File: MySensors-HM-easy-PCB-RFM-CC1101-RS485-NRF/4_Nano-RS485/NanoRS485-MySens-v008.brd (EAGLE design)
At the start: 25 x 38.7 mm, 47 parts, among them IC1 ATSHA204A, IC2 AT25DF512C-SSHN-B, IC3 REG1117, IC31 ATMEGA168-TQFP, X2 1751264, Y2 8MHZ

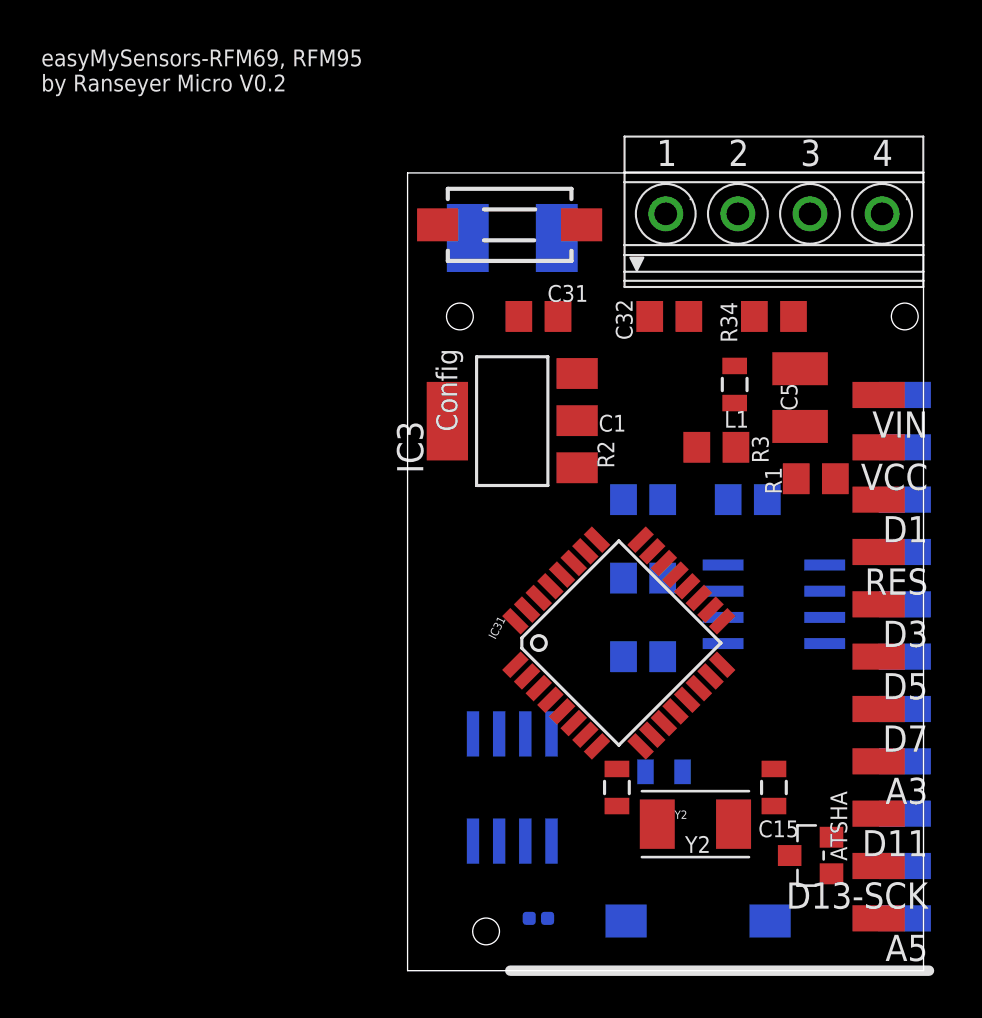
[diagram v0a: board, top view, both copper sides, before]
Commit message: update
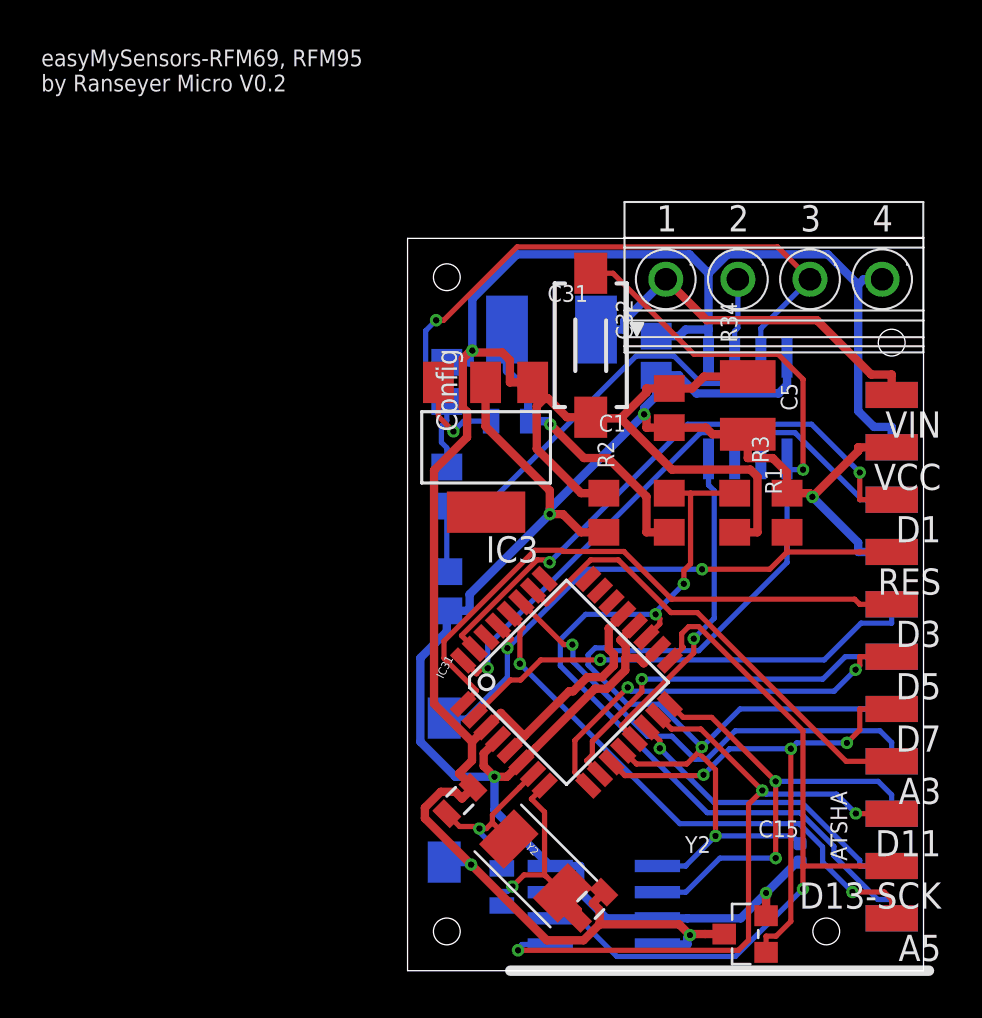
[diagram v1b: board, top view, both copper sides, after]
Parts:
- moved R7 15.7 mm to (1.91, 28.6), turned to 90 degrees
- moved C10 14.6 mm to (12.1, 29.8), turned to 270 degrees
- moved RESET 13.9 mm to (1.78, 8.76), turned to 90 degrees
- moved R2 13.1 mm to (19.1, 5.71), turned to 0 degrees
- moved L1 11.1 mm to (4.95, 26.7), flipped to the bottom, turned to 0 degrees
- moved C15 10.6 mm to (8.89, 3.17), turned to 225 degrees
- moved C32 10.0 mm to (9.53, 22.2), turned to 90 degrees
- moved R4 9.66 mm to (4.57, 4.06), turned to 90 degrees
- moved RS485 9.61 mm to (16.5, 27.3), turned to 90 degrees
- moved R5 9.55 mm to (1.91, 23.5), turned to 90 degrees
- moved R6 9.55 mm to (1.91, 18.4), turned to 90 degrees
- moved R34 9.55 mm to (18.4, 22.2), turned to 270 degrees
- moved Y2 8.01 mm to (6.22, 5.08), turned to 315 degrees
- moved C31 7.75 mm to (12.7, 27.3), turned to 90 degrees
- moved C14 7.65 mm to (2.54, 8.26), turned to 225 degrees
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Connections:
- removed net IN: F1.P$2
- removed net UREG: F1.P$1
- new net VIN-FUSED: F1.P$1, L1.1, R1.1
- net A: now also X2.2
- net B: now also X2.3
- net GND: now also X2.4
- net VIN: now also F1.P$2, X2.1; no longer L1.1, R1.1
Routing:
- net GND: track 0.00 -> 140.2 mm, vias 0 -> 3
- net VCC: track 0.00 -> 106.4 mm, vias 0 -> 5
- net D8: track 0.00 -> 68.5 mm, vias 0 -> 3
- net A6: track 0.00 -> 39.6 mm, vias 0 -> 2
- net D13_SCK: track 0.00 -> 36.1 mm, vias 0 -> 1
- net D11_MOSI: track 0.00 -> 34.0 mm, vias 0 -> 3
- net B: track 0.00 -> 33.5 mm, vias 0 -> 1
- net D2_INT0: track 0.00 -> 30.5 mm, vias 0 -> 1
- net D3: track 0.00 -> 28.6 mm
- net D1-TXD: track 0.00 -> 28.4 mm, vias 0 -> 2
- net RESET: track 0.00 -> 28.3 mm, vias 0 -> 2
- net A5: track 0.00 -> 26.9 mm, vias 0 -> 2
- net D7-ATSHA: track 0.00 -> 26.5 mm, vias 0 -> 3
- net A: track 0.00 -> 25.9 mm
- net D12_MISO: track 0.00 -> 23.7 mm, vias 0 -> 2
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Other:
- board size 25 x 38.7 mm -> 25 x 35.5 mm

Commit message: Update
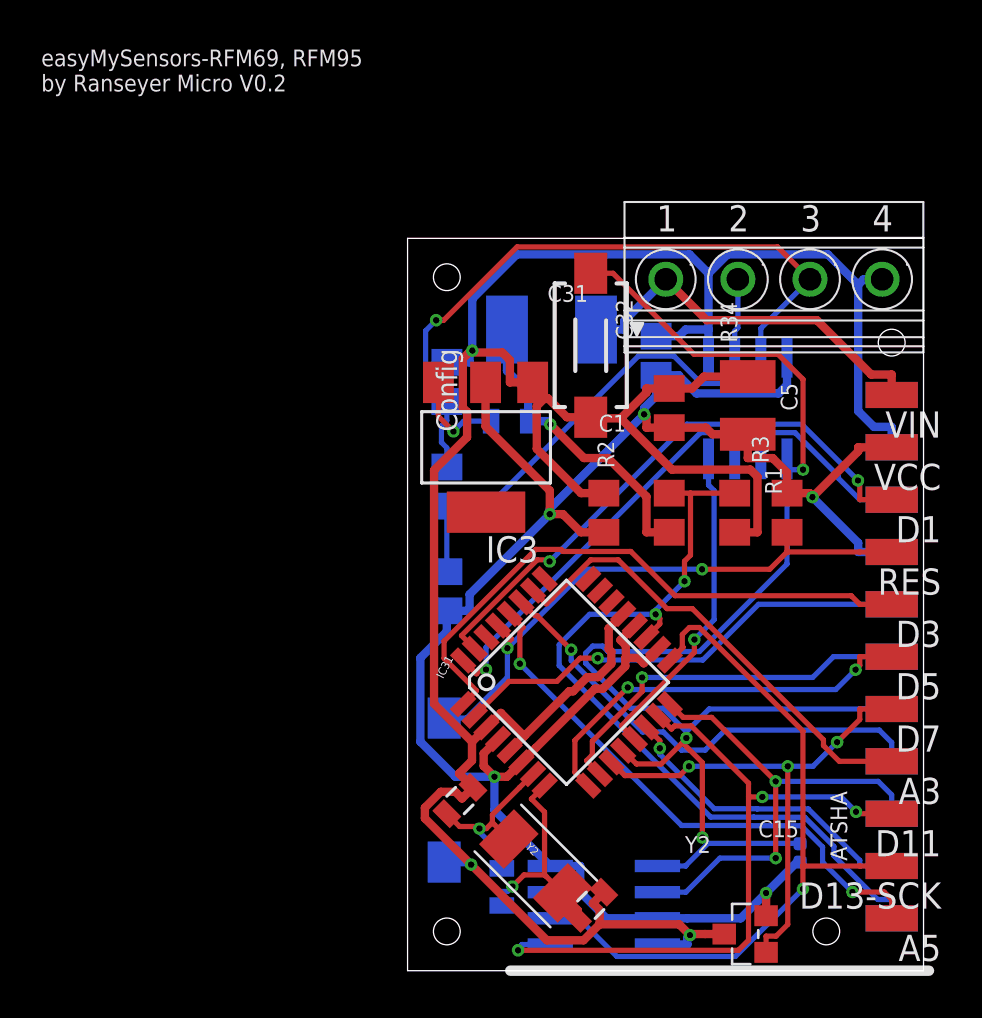
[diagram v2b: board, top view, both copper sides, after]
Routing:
- net D7-ATSHA: track 26.5 -> 25.3 mm
- net A4: track 23.3 -> 22.8 mm
